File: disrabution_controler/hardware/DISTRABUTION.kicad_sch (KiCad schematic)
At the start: 116 parts, among them Q1 PMOS, Q10 PMOS, Q11 PMOS, Q12 PMOS, Q13 PMOS, Q14 PMOS, Q15 PMOS, Q16 PMOS, Q2 PMOS, Q3 PMOS, Q4 PMOS, Q5 PMOS, Q6 PMOS, Q7 PMOS, Q8 PMOS, Q9 PMOS

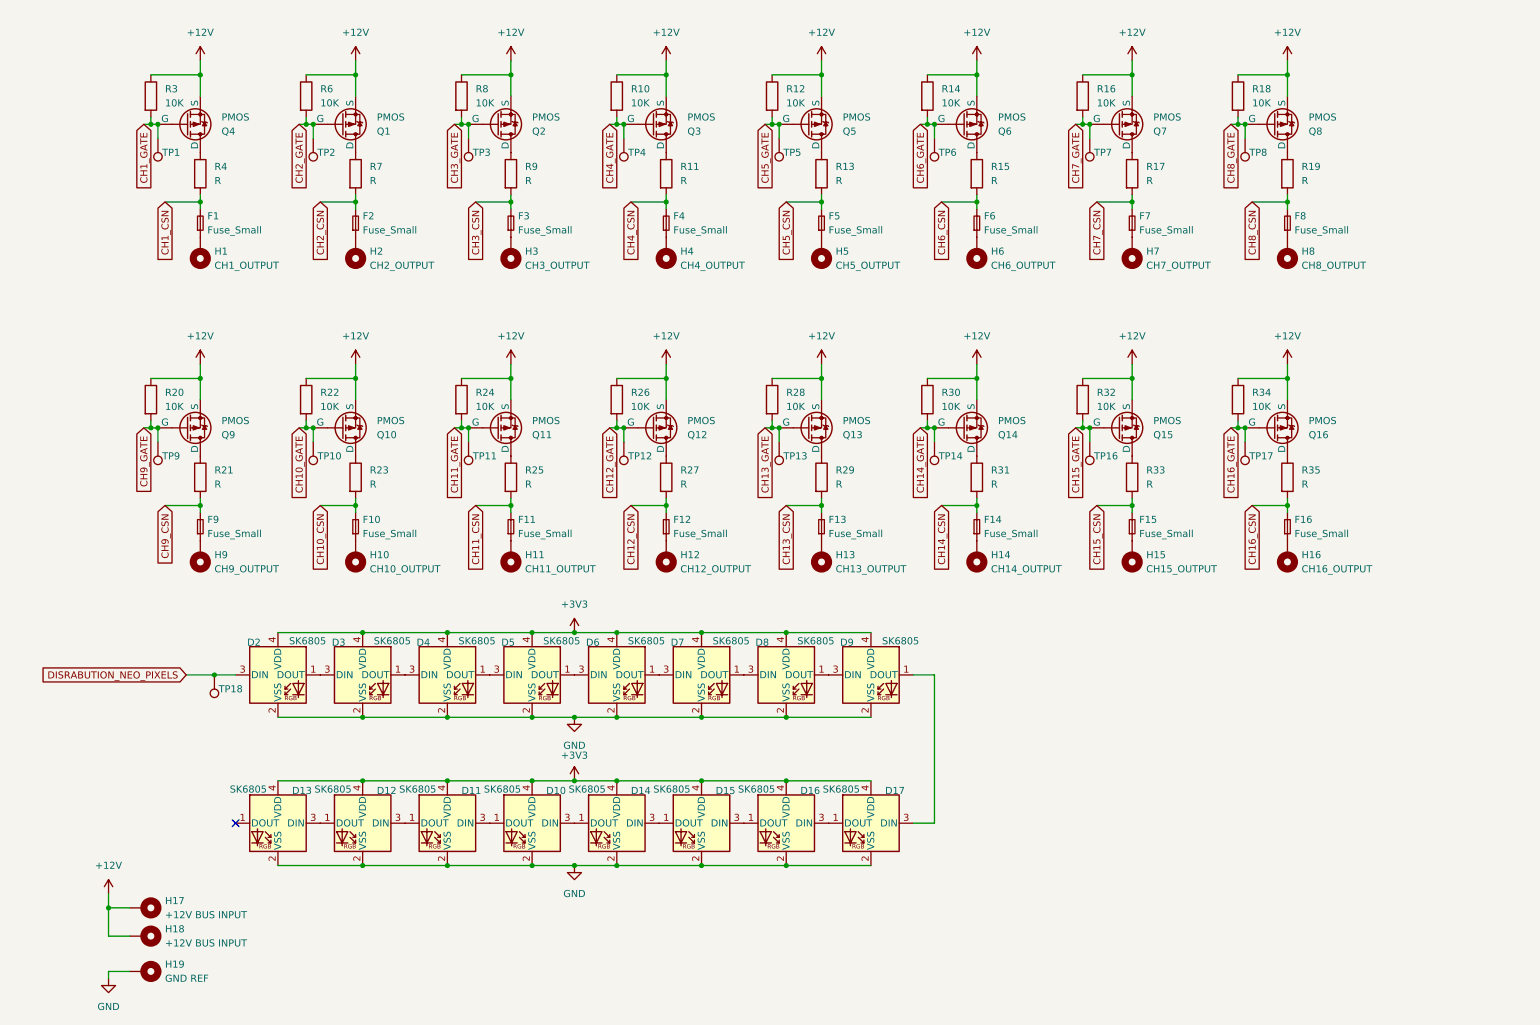
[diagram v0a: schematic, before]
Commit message: more hardware work
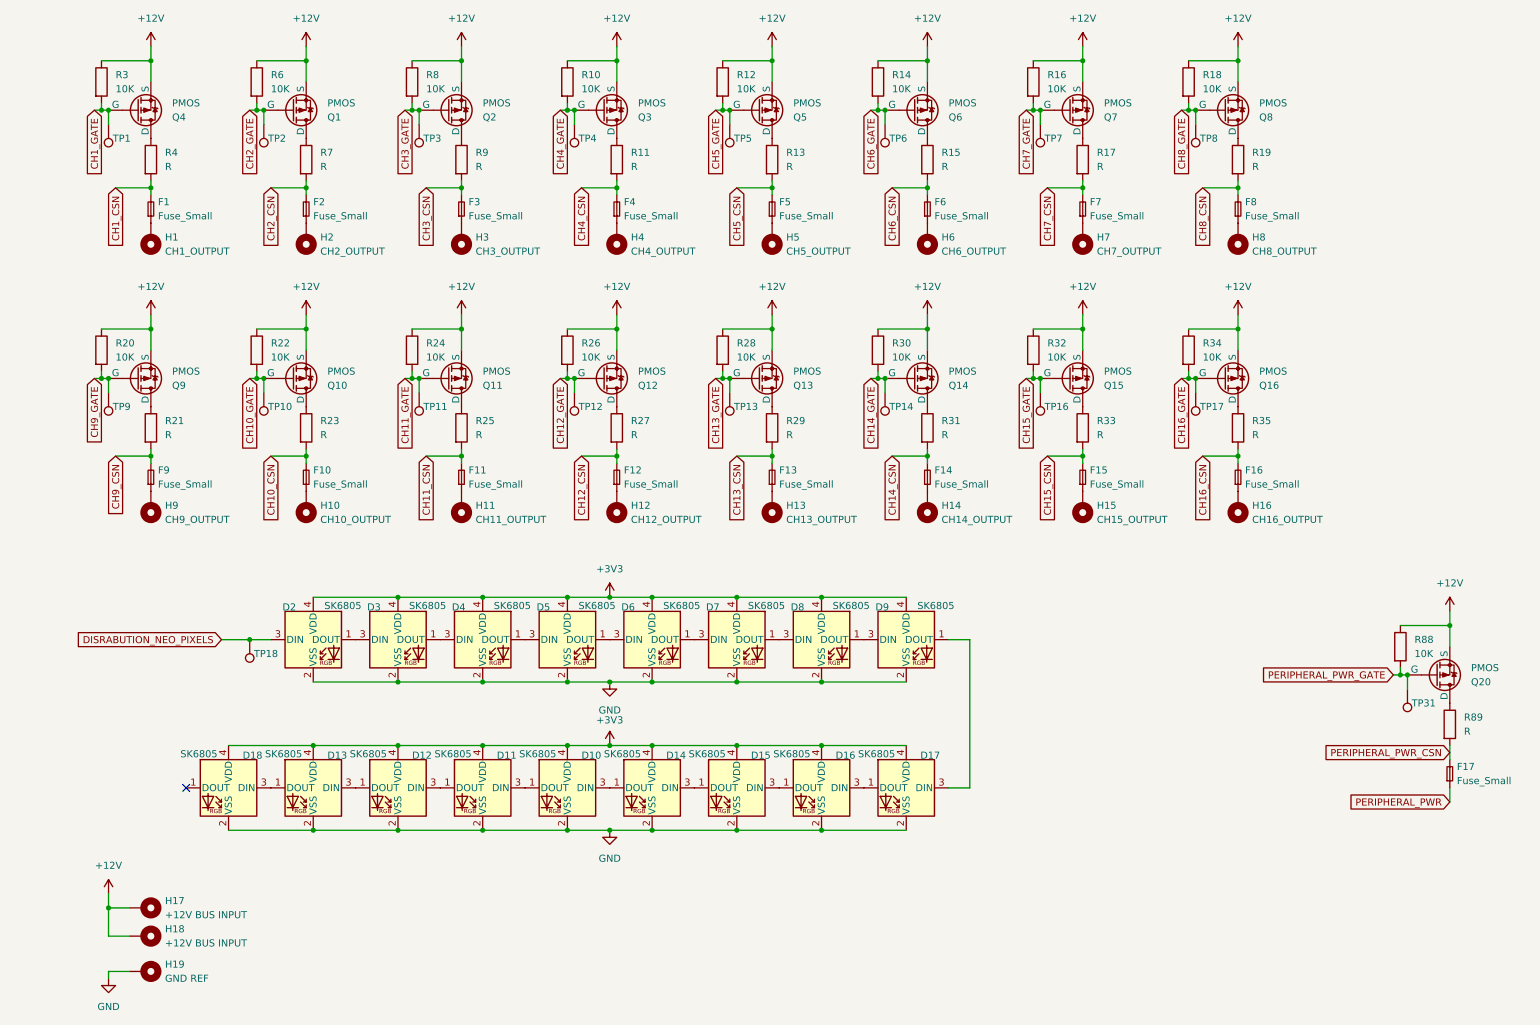
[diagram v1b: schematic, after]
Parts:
- added D18: SK6805, LED_SMD:LED_SK6805_PLCC4_2.4x2.7mm_P1.3mm, symbol LED:SK6805
- added F17: Fuse_Small, symbol Device:Fuse_Small
- added Q20: PMOS, symbol Simulation_SPICE:PMOS
- added R88: 10K, symbol Device:R
- added R89: R, symbol Device:R
- added TP31: ~, symbol Connector:TestPoint
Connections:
- net +12V: now also Q20.3 (S), R88.1
- net +3V3: now also D18.4 (VDD)
- net GND: now also D18.2 (VSS)
- net at D13.1 (DOUT): now also D18.3 (DIN)
- new net: Q20.1 (D), R89.1
- new net PERIPHERAL_PWR: F17.1
- new net PERIPHERAL_PWR_CSN: F17.2, R89.2
- new net PERIPHERAL_PWR_GATE: Q20.2 (G), R88.2, TP31.1
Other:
- moved on the sheet: D10, D11, D12, D13, D14, D15, D16, D17, D2, D3, D4, D5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
